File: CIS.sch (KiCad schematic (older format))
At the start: 181 parts, among them J1 K_9998, J2 RJ45_Abracon_ARJP11A-MASA-B-A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, J3 SJ1-3533NG, J4 DEBUG TAG, K1 K_9999, P3 K_0023, Q1 Q_0002, Q2 Q_0002, Q3 Q_0002, SW1 SW_0003, SW2 SW_0003, SW3 SW_0003, SW4 SW_0003, SW5 SW_0003, U1 U_0076, U14 U_0101, U16 U_0049, U17 U_0049, U2 STM32H745IIKx, U3 U_0103, U4 U_1001, U5 U_0081, U6 U_0097, U7 PCM5102, U8 ICM-20602

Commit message: Update libs WIP
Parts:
- removed C36: C_, DVB_Capacitors_Ceramic:C_0402, symbol DVB_C:C_0068
- removed C68, C69: C_, DVB_Capacitors_Ceramic:C_0402, symbol DVB_C:C_0001
- removed J1: K_9998, DVB_Connectors:Molex_PicoBlade_53261-1271_1x12-1MP_P1.25mm_Horizontal, symbol DVB_K:K_9998
- removed K1: K_9999, DVB_Displays:OLED256x64-2P1_HOLE_TE_3-2328724-1‎, symbol DVB_K:K_9999
- removed L2: L, DVB_Inductors:L_0402, symbol CIS-rescue:L-HM3-rescue
- removed L5: L_, DVB_Inductors:L_0603, symbol CIS-rescue:L_0010-HM3-rescue
- removed L6: L_, DVB_Inductors:L_4018-Coilcraft, symbol DVB_L:L_0011
- removed R50, R51: R_, DVB_Resistors:R_0402, symbol DVB_R:R_0075
- added C36: C_0080, DVB_Capacitors_Ceramic:C_0402, symbol DVB_C:C_0080
- added C68, C69: C_0064, DVB_Capacitors_Ceramic:C_0402, symbol DVB_C:C_0064
- added K1: K_0073, DVB_Displays:OLED256x64-2P1_HOLE_TE_3-2328724-1‎, symbol DVB_K:K_0073
- added K2: K_0072, DVB_Connectors:Molex_PicoBlade_53261-1271_1x12-1MP_P1.25mm_Horizontal, symbol DVB_K:K_0072
- added L2: L_0016, DVB_Inductors:L_0402, symbol DVB_L:L_0016
- added L5: L_0017, DVB_Inductors:L_0603, symbol DVB_L:L_0017
- added L6: L_0018, DVB_Inductors:L_4018-Coilcraft, symbol DVB_L:L_0018
- added R50, R51: R_0169, DVB_Resistors:R_0402, symbol DVB_R:R_0169
- C1, C10, C12, C19, C2, C29, C3, C32, C33, C34, C38, C40, C42, C52, C53, C56, C57, C58, C59, C6, C62, C65, C67, C70, C78, C79, C8, C82, C84, C86, C87: symbol CIS-rescue:C_0002-HM3-rescue -> DVB_C:C_0002; Field1 100nF -> (none); Field2 C-0402 -> (none); Field3 25V -> (none); Field4 25V -> CER; Field5 (none) -> 100nF; Field6 (none) -> 25V; Field7 (none) -> X7R; Field8 (none) -> 10%
- C14, C43, C44, C45, C47, C49, C54, C55, C89, C91: symbol CIS-rescue:C_0002-HM3-rescue -> DVB_C:C_0002; Field1 100nF -> (none); Field2 C-0402 -> (none); Field3 25V -> (none); Field4 X7R -> CER; Field5 (none) -> 100nF; Field6 (none) -> 25V; Field7 (none) -> X7R; Field8 (none) -> 10%
- C17, C21, C22, C23: symbol CIS-rescue:C_0043-HM3-rescue -> DVB_C:C_0043; Field1 18pF -> (none); Field2 C-0402 -> (none); Field3 50V -> (none); Field4 C0G/N0P -> CER; Field5 (none) -> 18pF; Field6 (none) -> 50V; Field7 (none) -> COG/NPO; Field8 (none) -> 5%
- C39: symbol CIS-rescue:C_0036-HM3-rescue -> DVB_C:C_0036; Field1 470pF -> (none); Field2 C-0603 -> (none); Field3 25V -> (none); Field4 X5R -> CER; Field5 (none) -> 4.7µF; Field6 (none) -> 25V; Field7 (none) -> X5R; Field8 (none) -> 10%
- C4, C46, C5, C9: symbol CIS-rescue:C_0003-HM3-rescue -> DVB_C:C_0003; Field1 10uF -> (none); Field2 C-0603 -> (none); Field3 25V -> (none); Field4 X5R -> CER; Field5 (none) -> 10µF; Field6 (none) -> 25V; Field7 (none) -> X5R; Field8 (none) -> 10%
- C63, C64, C75, C76: symbol CIS-rescue:C_0045-HM3-rescue -> DVB_C:C_0045; Field1 2.2uF -> (none); Field2 C-0402 -> (none); Field3 25V -> (none); Field4 X5R -> CER; Field5 (none) -> 2.2µF; Field6 (none) -> 25V; Field7 (none) -> X5R; Field8 (none) -> 10%
- D1: symbol CIS-rescue:D_0001-HM3-rescue -> DVB_D:D_0001; Field1 TLMS1000-GS08 -> (none); Field2 LED-0603 -> (none); Field3 LED -> (none); Field4 2.6V -> TLMS1000-GS08; Field6 4mcd -> LED
- D6: symbol CIS-rescue:D_0020-HM3-rescue -> DVB_D:D_0020; Field1 CD0603-B0230 -> (none); Field2 D_0603 -> (none); Field3 SCHOTTKY -> (none); Field4 30V -> CD0603-B0240R; Field6 0.5Vf -> SCHOTTKY; Field7 12pF -> 1-Chan; Field8 1-Chan -> 30Vr
- J2: footprint DVB_Connectors:RJ45_Abracon_ARJP11A-MA_Horizontal -> Connector_RJ:RJ45_Abracon_ARJP11A-MA_Horizontal
- J3: footprint DVB_Connectors:Jack_3.5mm_CUI_SJ1-3533NG_Horizontal -> (none)
- J4: footprint Connector:Tag-Connect_TC2030-IDC-NL_2x03_P1.27mm_Vertical -> (none)
- P3: footprint DVB_Connectors:SHF-105-01-L-D-TH -> DVB_Connectors:SHF-105-01-L-D-RA; symbol CIS-rescue:K_0023-HM3-rescue -> DVB_K:K_0023; Field1 SHF-105-01-L-D -> (none); Field2 SHF-105-01-L-D-RA -> (none); Field3 Samtec -> (none); Field4 10p -> SHF-105-01-L-D-RA; Field5 5ppr -> 10p; Field6 350mA -> fem; Field7 fem -> RA; Field8 null -> (none)
- Q1, Q2, Q3: Field1 N-chan -> BSS138PW
- R1, R21, R22, R32, R33, R36, R39, R4, R42, R43, R46, R47, R53: symbol CIS-rescue:R_0020-HM3-rescue -> DVB_R:R_0020; Field1 10K -> (none); Field2 R-0402 -> (none); Field3 1% -> (none); Field4 100mW -> 10k; Field5 (none) -> 1%; Field6 (none) -> 100mW
- R10, R11, R52: symbol CIS-rescue:R_0020-HM3-rescue -> DVB_R:R_0020; Field1 NC -> (none); Field2 R-0402 -> (none); Field4 (none) -> 10k; Field5 (none) -> 1%; Field6 (none) -> 100mW
- R16: symbol CIS-rescue:R_0104-HM3-rescue -> DVB_R:R_0104; Field1 750 -> (none); Field2 R-0402 -> (none); Field3 1% -> (none); Field4 63mW -> 750; Field5 (none) -> 1%; Field6 (none) -> 63mW
- R17: Field4 12.1K -> 12.1k
- R23: Field4 130 -> 36k
- R25: Field4 75 -> 36k
- R28, R29, R30, R31: Field4 49.9K -> 49.9k
- R38: symbol CIS-rescue:R_0118-HM3-rescue -> DVB_R:R_0018; Field1 1.5K -> (none); Field2 R-0402 -> (none); Field3 1% -> (none); Field4 62.5mW -> 7.15k; Field5 (none) -> 1%; Field6 (none) -> 100mW
- R44: Field4 68 -> 36k
- U14: symbol CIS-rescue:U_0101-HM3-rescue -> DVB_U:U_0101
- U16, U17: symbol CIS-rescue:U_0049-HM3-rescue -> DVB_U:U_0049; Field1 CD143A-SR3.3 -> (none); Field3 Bourns -> (none); Field4 ESD -> CD143A-SR3.3; Field5 0 -> PROTECTION; Field6 0 -> ESD / D-ARRAY; Field7 0 -> 2-Chan
- U4: Field4 LT8610AEMSE-3.3 -> LT8610ABIMSE-5
- U8: footprint DVB_LGA:LGA-16_3x3mm_P0.5mm_LayoutBorder3x5y -> Package_LGA:LGA-16_3x3mm_P0.5mm_LayoutBorder3x5y
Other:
- note added: "A rationnaliser avec L7 en 0603"
- note removed: "optional\n0ohm\nor bead\n600R@100MHz"

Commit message: Update libs
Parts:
- removed R23, R25, R44: R_, DVB_Resistors:R_0402, symbol DVB_R:R_0130
- removed U2: STM32H745IIKx, DVB_BGA:UFBGA_176, symbol DVB_U:STM32H745IIKx
- removed U7: PCM5102, Package_SO:TSSOP-20_4.4x6.5mm_P0.65mm, symbol Audio:PCM5102
- removed U8: ICM-20602, Package_LGA:LGA-16_3x3mm_P0.5mm_LayoutBorder3x5y, symbol Sensor_Motion:ICM-20602
- added R23: R_0170, DVB_Resistors:R_0402, symbol DVB_R:R_0170
- added R25: R_0171, DVB_Resistors:R_0402, symbol DVB_R:R_0171
- added R44: R_0172, DVB_Resistors:R_0402, symbol DVB_R:R_0172
- added U2: U_0131, DVB_BGA:UFBGA_176, symbol DVB_U:U_0131
- added U7: U_0132, DVB_SSOP:TSSOP-20_4.4x6.5mm_P0.65mm, symbol DVB_U:U_0132
- added U8: U_0133, DVB_LGA:LGA-16_3x3mm_P0.5mm_LayoutBorder3x5y, symbol DVB_U:U_0133
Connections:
- net +3.3V: now also U2.D11 (VDD), U2.D5 (VDD), U2.E12 (VDD), U2.E15 (VDD50_USB), U2.E2 (VBAT), U2.E4 (VDD), U2.F13 (VDD33_USB), U2.G4 (VDD), U2.H12 (VDD), U2.K4 (VDD), U2.L12 (VDD), U2.M5 (VDD), U2.M9 (VDD), U7.1 (CPVDD), U7.20 (DVDD), U7.8 (AVDD), U8.1 (VDDIO), U8.16 (VDD)
- net 12V_EN: now also U2.F15 (PG5)
- net 5V_EN: now also U2.G15 (PG2)
- net CIS_ADC_1: now also U2.R3 (PA0_C)
- net CIS_ADC_2: now also U2.P3 (PA1_C)
- net CIS_ADC_3: now also U2.N2 (PC3_C)
- net CIS_CP: now also U2.D13 (PA9)
- net CIS_LED_B: now also U2.E14 (PC6)
- net CIS_LED_G: now also U2.N15 (PH12)
- net CIS_LED_R: now also U2.H15 (PD13)
- net CIS_RS: now also U2.B15 (PA12)
- net CIS_SP: now also U2.D14 (PC8)
- net CIS_VLED_B: now also R44.1
- net CIS_VLED_G: now also R25.1
- net CIS_VLED_R: now also R23.1
- net DAC_BCK: now also U2.D3 (PE5), U7.13 (BCK)
- net DAC_DEMP: now also U2.R4 (PH3), U7.10 (DEMP)
- net DAC_DIN: now also U2.D9 (PD6), U7.14 (DIN)
- net DAC_FLT: now also U2.C1 (PC13), U7.11 (FLT)
- net DAC_FMT: now also U2.H1 (PF6), U7.16 (FMT)
- net DAC_LRCK: now also U2.B1 (PE4), U7.15 (LRCK)
- net DAC_SCK: now also U2.C3 (PE2), U7.12 (SCK)
- net DAC_XSMT: now also U2.M1 (PC2), U7.17 (XSMT)
- net DEBUG_RX: now also U2.B5 (PB7)
- net DEBUG_TX: now also U2.A5 (PB6)
- net FMC_Ax: now also U2.F4 (PF0)
- net FMC_D0: now also U2.H14 (PD14)
- net FMC_D1: now also U2.J12 (PD15)
- net FMC_D2: now also U2.C10 (PD0)
- net FMC_D3: now also U2.A10 (PD1)
- net FMC_D4: now also U2.P9 (PE7)
- net FMC_D5: now also U2.N8 (PE8)
- net FMC_D6: now also U2.R11 (PE9)
- net FMC_D7: now also U2.R9 (PE10)
- net FMC_NEx: now also U2.B8 (PD7)
- net FMC_NOE: now also U2.C9 (PD4)
- net FMC_NWE: now also U2.B9 (PD5)
- net GND: now also U2.A1 (VSS), U2.A15 (VSS), U2.C2 (VSS), U2.D10 (VSS), U2.D6 (VSS), U2.E1 (VSS), U2.F10 (VSS), U2.F12 (VSS), U2.F2 (VSSSMPS), U2.F6 (VSS), U2.F7 (VSS), U2.F8 (VSS), U2.F9 (VSS), U2.G10 (VSS), U2.G6 (VSS), U2.G7 (VSS), U2.G8 (VSS), U2.G9 (VSS), U2.H10 (VSS), U2.H6 (VSS), U2.H7 (VSS), U2.H8 (VSS), U2.H9 (VSS), U2.J10 (VSS), U2.J14 (VSS), U2.J6 (VSS), U2.J7 (VSS), U2.J8 (VSS), U2.J9 (VSS), U2.K10 (VSS), U2.K12 (VSS), U2.K2 (VSS), U2.K6 (VSS), U2.K7 (VSS), U2.K8 (VSS), U2.K9 (VSS), U2.M10 (VSS), U2.M6 (VSS), U2.N3 (VSSA), U2.R1 (VSS), U2.R15 (VSS), U7.19 (DGND), U7.3 (CPGND), U7.9 (AGND), U8.10 (GND), U8.11 (GND), U8.12 (GND), U8.13 (GND), U8.15 (GND), U8.9 (GND)
- net LED1: now also U2.P15 (PH6)
- net MEMS_CS: now also U2.B3 (PB9), U8.5 (~CS)
- net MEMS_FSYNC: now also U2.A11 (PA15), U8.8 (FSYNC)
- net MEMS_INT: now also U2.L14 (PD8), U8.6 (INT)
- net MEMS_MISO: now also U2.K15 (PB14), U8.4 (SAO/SD0)
- net MEMS_MOSI: now also U2.K14 (PB15), U8.3 (SDA/SDI)
- net MEMS_SCLK: now also U2.A9 (PD3), U8.2 (SCL/SPC)
- net OLED_RESET: now also U2.A2 (PB8)
- net RMII_CRS_DV: now also U2.N6 (PA7)
- net RMII_MDC: now also U2.L3 (PC1)
- net RMII_MDIO: now also U2.R2 (PA2)
- net RMII_REF_CLK: now also U2.P2 (PA1)
- net RMII_RXD0: now also U2.R6 (PC4)
- net RMII_RXD1: now also U2.M7 (PC5)
- net RMII_TXD0: now also U2.B7 (PG13)
- net RMII_TXD1: now also U2.C7 (PG14)
- net RMII_TX_EN: now also U2.A7 (PG11)
- net RST: now also U2.L1 (NRST)
- net SWD-CLK: now also U2.A12 (PA14)
- net SWD-IO: now also U2.B13 (PA13)
- net SW_DOWN: now also U2.P13 (PE13)
- net SW_LEFT: now also U2.M12 (PE14)
- net SW_OK: now also U2.P14 (PE15)
- net SW_RIGHT: now also U2.P12 (PE12)
- net SW_UP: now also U2.R12 (PE11)
- net VERF+: now also U2.M3 (VREF+)
- net VERF-: now also U2.L4 (VREF-)
- net at C23.2, XO2.3: now also U2.K1 (PH1)
- net at C22.1, XO2.1: now also U2.J1 (PH0)
- net at R4.1, R52.2: now also U2.C5 (BOOT0)
- net at C67.2: now also U7.18 (LDOO)
- net at C63.2: now also U7.2 (CAPP)
- net at C63.1: now also U7.4 (CAPM)
- net at C64.2: now also U7.5 (VNEG)
- net at R50.1: now also U7.6 (OUTL)
- net at R51.2: now also U7.7 (OUTR)
- net at C71.2, L5.1: now also U2.G1 (VDDSMPS)
- net at C72.1, C73.1, C74.1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: now also U2.A13 (VDDLO), U2.A14 (VCAP), U2.A3 (VDDLO), U2.A4 (VCAP), U2.G2 (VFBSMPS), U2.R13 (VCAP), U2.R14 (VDDLO)
- net at R53.2: now also U2.D4 (PDR_ON)
- net at C36.1, L6.2: now also U2.F1 (VLXSMPS)
- net at C81.2, C82.1, L7.2: now also U2.M4 (VDDA)
- net at C70.2: now also U8.14 (REGOUT)
- net at Q1.3 (D): now also R23.2
- net at Q2.3 (D): now also R25.2
- net at Q3.3 (D): now also R44.2

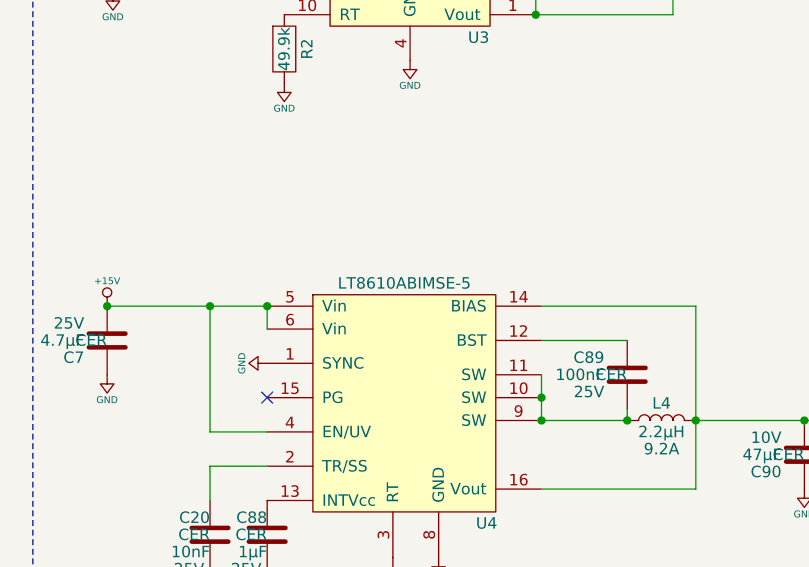
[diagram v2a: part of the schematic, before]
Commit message: Update pos files
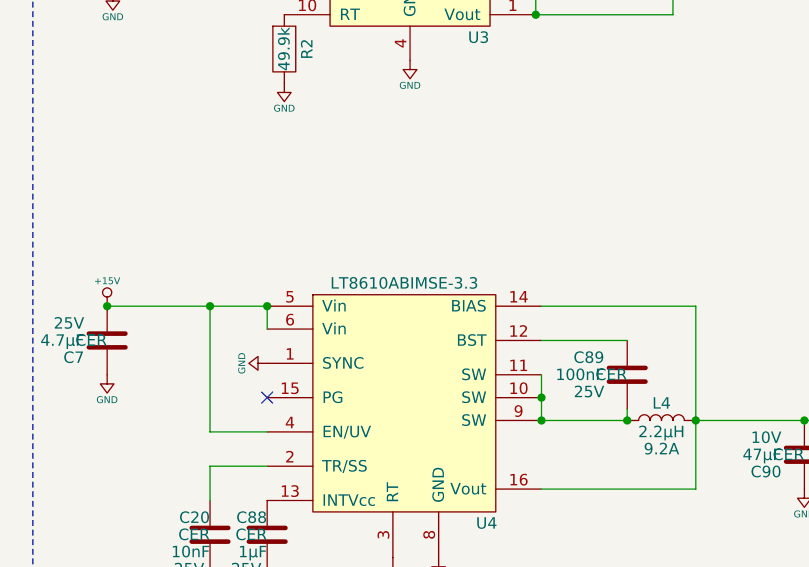
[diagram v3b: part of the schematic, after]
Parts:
- removed U4: U_1001, DVB_SSOP:MSOP_16-1EP_3x4_P0.5, symbol DVB_U:U_0065
- added U4: U_0134, DVB_SSOP:MSOP_16-1EP_3x4_P0.5, symbol DVB_U:U_0134
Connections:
- net +15: now also U4.4 (EN/UV), U4.5 (Vin), U4.6 (Vin)
- net +3.3V: now also U4.14 (BIAS), U4.16 (Vout)
- net GND: now also U4.1 (SYNC), U4.17 (GND), U4.8 (GND)
- net at C89.2, L4.1: now also U4.10 (SW), U4.11 (SW), U4.9 (SW)
- net at C89.1: now also U4.12 (BST)
- net at C88.2: now also U4.13 (INTVcc)
- net at C20.2: now also U4.2 (TR/SS)
- net at R3.1: now also U4.3 (RT)
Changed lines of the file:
@@
 Connection ~ 3575 13325
 Wire Wire Line
-	2925 11350 2925 11450
-Connection ~ 2925 11450
-Wire Wire Line
-	2925 11450 2925 11550
-Wire Wire Line
 	2925 11550 3300 11550
 Wire Wire Line
 	3300 11550 3300 11500
-Connection ~ 2925 11550
 Connection ~ 3300 11550
 Wire Wire Line
@@
 Wire Wire Line
 	1725 11150 1725 11050
-Connection ~ 1725 11050
 Wire Wire Line
 	1025 11050 1475 11050
@@
 $EndComp
 $Comp
-L DVB_U:U_0065 U4
-U 1 1 5FFDF071
-P 2325 11500
-F 0 "U4" H 2685 11000 50  0000 C CNN
-F 1 "U_1001" H 2275 10750 50  0001 C CNN
-F 2 "DVB_SSOP:MSOP_16-1EP_3x4_P0.5" H 2275 10650 50  0001 C CNN
-F 3 "http://cds.linear.com/docs/en/datasheet/8610abfa.pdf" H 2275 10550 50  0001 C CNN
-F 4 "LT8610ABIMSE-5" H 2325 12050 50  0000 C CNN "Field4"
-F 5 "REGULATOR" H 2325 9960 50  0001 C CNN "Field5"
-F 6 "DC/DC BUCK" H 2275 10450 50  0001 C CNN "Field6"
-F 7 "3.4V to 42Vcc" H 2275 10350 50  0001 C CNN "Field7"
-F 8 "5Vout" H 2275 10250 50  0001 C CNN "Field8"
-F 9 "3.5A" H 2275 10150 50  0001 C CNN "Field9"
-	1    2325 11500
-	1    0    0    -1
-$EndComp
-$Comp
 L DVB_C:C_0002 C89
 U 1 1 5FFE3EA7
@@
 $EndComp
 Connection ~ 11025 9600
+$Comp
+L DVB_U:U_0134 U4
+U 1 1 605CB444
+P 2325 11500
+F 0 "U4" H 2685 11000 50  0000 C CNN
+F 1 "U_0134" H 2275 10750 50  0001 C CNN
+F 2 "DVB_SSOP:MSOP_16-1EP_3x4_P0.5" H 2275 10650 50  0001 C CNN
+F 3 "http://cds.linear.com/docs/en/datasheet/8610abfa.pdf" H 2275 10550 50  0001 C CNN
+F 4 "LT8610ABIMSE-3.3" H 2325 12050 50  0000 C CNN "Field4"
+F 5 "REGULATOR" H 2325 9960 50  0001 C CNN "Field5"
+F 6 "DC/DC BUCK" H 2275 10450 50  0001 C CNN "Field6"
+F 7 "3.4V to 42Vcc" H 2275 10350 50  0001 C CNN "Field7"
+F 8 "3.3Vout" H 2275 10250 50  0001 C CNN "Field8"
+F 9 "3.5A" H 2275 10150 50  0001 C CNN "Field9"
+	1    2325 11500
+	1    0    0    -1
+$EndComp
+Wire Wire Line
+	2925 11350 2925 11450
+Connection ~ 1725 11050
+Wire Wire Line
+	2925 11450 2925 11550
+Connection ~ 2925 11450
+Connection ~ 2925 11550
 $EndSCHEMATC
